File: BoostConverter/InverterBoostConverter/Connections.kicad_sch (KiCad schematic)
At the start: 17 parts, among them J1 1987724, J2 1987724, J3 Conn_Coaxial, J4 Conn_Coaxial, J5 Conn_01x02_Pin, J6 Conn_01x02_Pin, M1 Fan_4pin

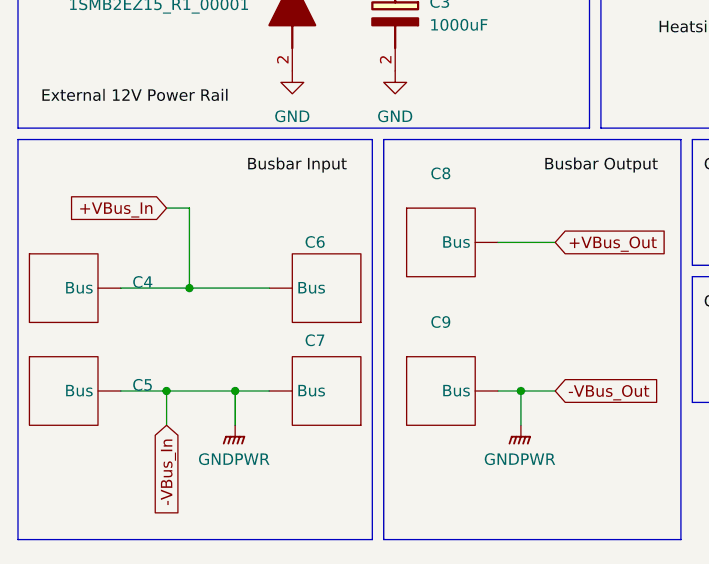
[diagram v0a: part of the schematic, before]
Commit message: Finish Boost Converter
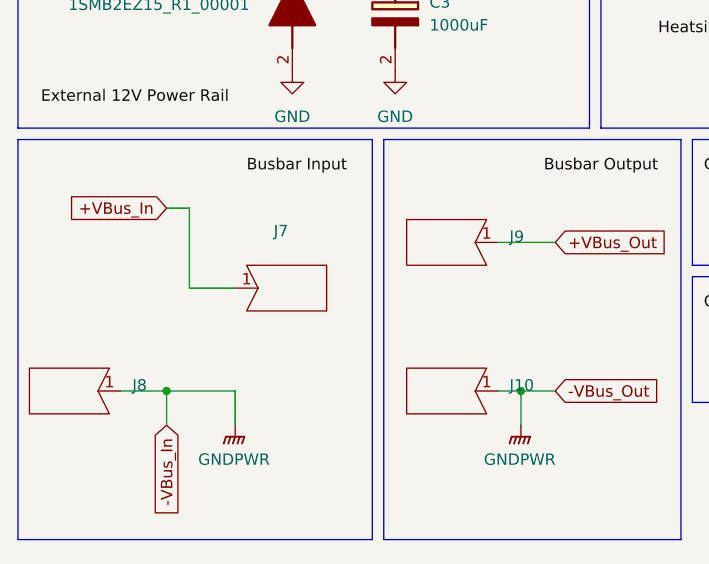
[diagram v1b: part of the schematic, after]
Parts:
- removed C4, C5, C6, C7, C8, C9: ~, symbol InverterCom:BusBarConnection
- added J10, J7, J8, J9: ~, InverterCom:WireSolderJoint, symbol InverterCom:WireSolderJoint
- C2, C3: footprint CAPPRD500W60D1025H1750 -> InverterCom:CAPPRD500W60D1025H1750
- J1, J2: footprint 1987724 -> InverterCom:1987724
- J3, J4: footprint (none) -> Connector_Coaxial:SMA_Wurth_60312002114503_Vertical
- J5, J6: footprint (none) -> Connector_PinSocket_2.54mm:PinSocket_1x02_P2.54mm_Vertical
- M1: footprint (none) -> Connector:FanPinHeader_1x04_P2.54mm_Vertical
- R61: footprint 1210 -> Resistor_SMD:R_1210_3225Metric_Pad1.30x2.65mm_HandSolder
- Z1: footprint 1SMB2EZ15_R1_00001 -> InverterCom:1SMB2EZ15_R1_00001
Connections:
- net +VBus_In: now also J7.1
- net +VBus_Out: now also J9.1
- net GNDPWR: now also J10.1, J8.1
